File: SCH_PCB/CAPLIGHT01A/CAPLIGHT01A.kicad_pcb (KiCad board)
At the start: 2 copper layers, 76.2 x 20.3 mm, 25 parts, among them J1 JUMP_3X2, J10 JUMP_2x1, J11 JUMP_3X2, J5 CONN1_1, J6 CONN1_1, J9 JUMP_2x1, P1 USB_OTG, U1 LTC3625

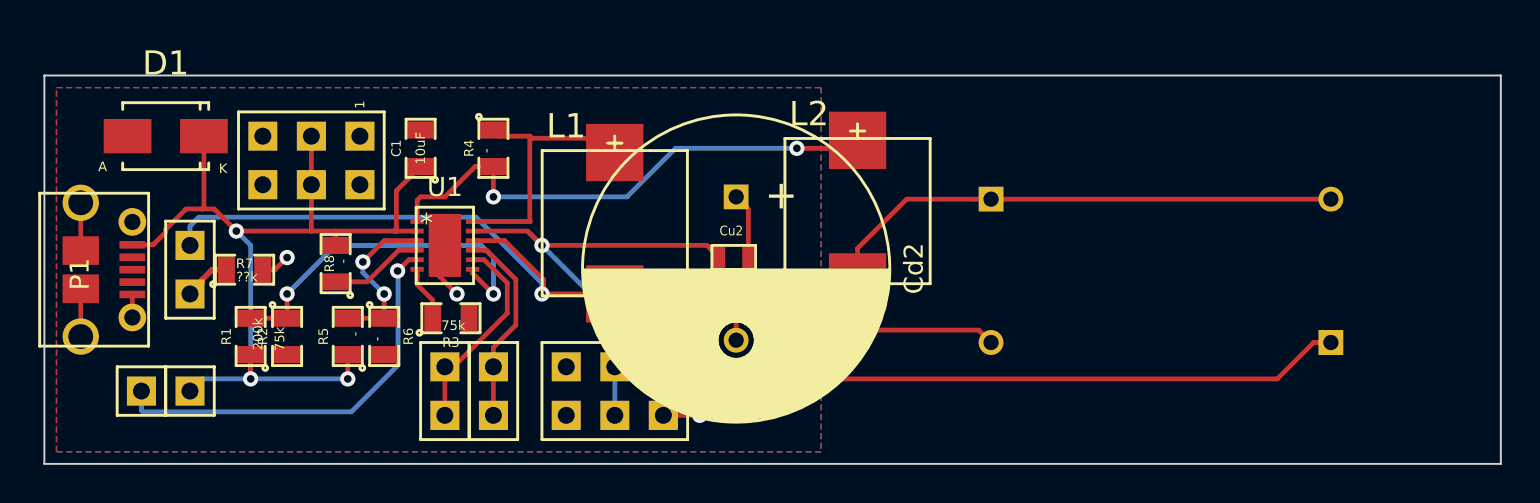
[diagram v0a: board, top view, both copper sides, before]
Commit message: only for ExpaLight
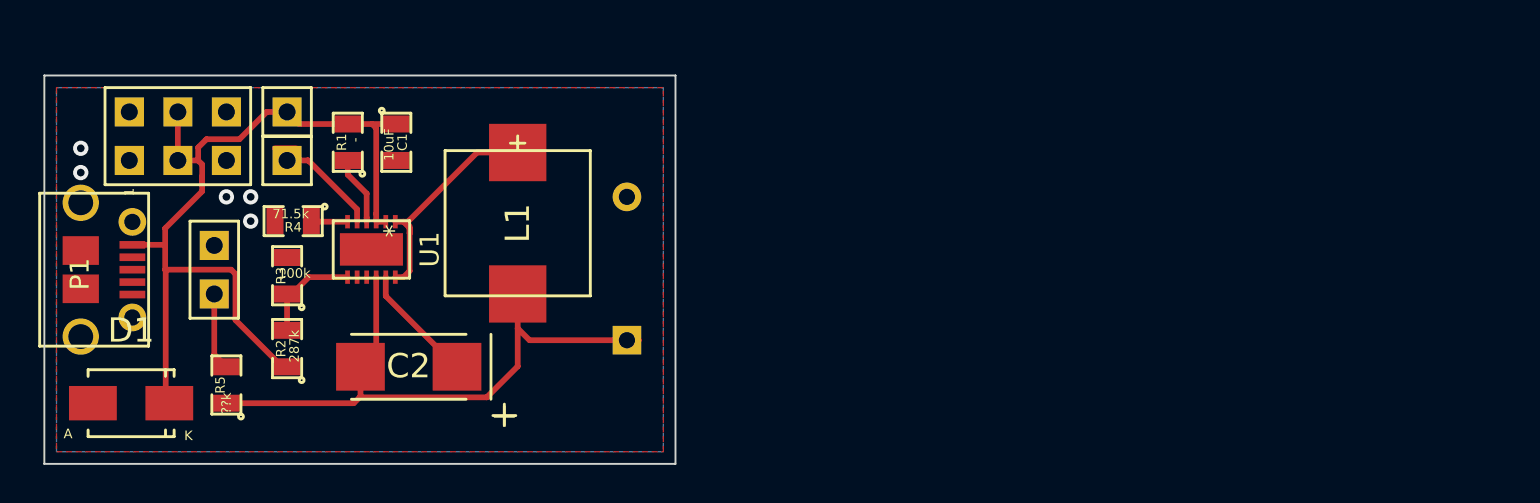
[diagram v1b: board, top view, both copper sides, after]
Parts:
- removed Cd1, Cd2, Cu1: 22F, Mlab_C:C_Radial_D16_L25_P7.5
- removed Cu2: 100uF, Mlab_C:SMD-0603
- removed J10, J9: JUMP_2x1, Mlab_Pin_Headers:Straight_2x01
- removed J11: JUMP_3X2, Mlab_Pin_Headers:Straight_2x03
- removed J5, J6: CONN1_1, Mlab_Pin_Headers:Straight_1x01
- removed L2: DER0705-3.3uH, Mlab_L:DER0705
- removed R6, R8: -, Mlab_R:SMD-0805
- removed R7: ??k, Mlab_R:SMD-0805
- added C2: 100uF, Mlab_C:TantalC_SizeC_Reflow, F.Cu at (156.9, 123.2)
- added C3: 22F, Mlab_C:C_Radial_D18_L25_P7.5, B.Cu at (168.3, 121.8)
- added J2: CONN1_1, Mlab_Pin_Headers:Straight_1x01, F.Cu at (150.5, 109.9)
- added J3: CONN1_1, Mlab_Pin_Headers:Straight_1x01, F.Cu at (150.5, 112.4)
- R1: value 200k -> -
- R2: value 75k -> 287k
- R3: value 75k -> 100k
- R4: value - -> 71.5k
- R5: value - -> ??k
- moved D1 14.1 mm to (142.3, 125.1)
- moved R1 11.4 mm to (153.7, 111.4)
- moved R4 11.1 mm to (150.8, 115.6), turned to 180 degrees
- moved R3 8.86 mm to (150.5, 118.4), turned to 90 degrees
- moved J1 7.10 mm to (144.8, 111.1), turned to 90 degrees
- moved R5 6.84 mm to (147.3, 124.1)
- moved L1 5.08 mm to (162.6, 115.7)
- moved U1 3.85 mm to (154.9, 117.0), turned to 270 degrees
- moved C1 1.31 mm to (156.2, 111.4), turned to 270 degrees
- moved D2 1.27 mm to (146.7, 118.1), turned to 0 degrees
- moved R2 0.63 mm to (150.5, 122.2), turned to 90 degrees
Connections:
- D2 pad 1: Net-(D2-Pad1) -> GND
- D2 pad 2: Net-(Cd1-Pad1) -> Net-(D2-Pad2)
- L1 pad 2: Net-(Cd1-Pad1) -> Net-(C2-Pad2)
- R1 pad 1: /VIN -> Net-(R1-Pad1)
- R1 pad 2: Net-(R1-Pad2) -> /VIN
- R2 pad 1: Net-(R1-Pad2) -> /VIN
- R2 pad 2: GND -> Net-(R2-Pad2)
- R3 pad 1: Net-(R3-Pad1) -> Net-(R2-Pad2)
- R4 pad 1: Net-(L1-Pad1) -> Net-(R4-Pad1)
- R4 pad 2: Net-(L2-Pad1) -> GND
- R5 pad 1: /VIN -> Net-(C2-Pad2)
- R5 pad 2: Net-(R5-Pad2) -> Net-(D2-Pad2)
- U1 pad 1: Net-(L2-Pad1) -> Net-(L1-Pad1)
- U1 pad 10: Net-(Cd1-Pad1) -> Net-(C2-Pad2)
- U1 pad 3: Net-(R5-Pad2) -> /VIN
- U1 pad 4: Net-(R8-Pad1) -> Net-(R1-Pad1)
- U1 pad 6: Net-(R3-Pad1) -> Net-(R4-Pad1)
- U1 pad 7: Net-(R1-Pad2) -> Net-(R2-Pad2)
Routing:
- net Net-(Cd1-Pad1): track 76.0 -> 0.00 mm, vias 1 -> 0
- net Net-(C2-Pad1): track 64.7 -> 6.25 mm, vias 2 -> 0
- net Net-(C2-Pad2): track 0.00 -> 33.0 mm
- net GND: track 29.8 -> 0.00 mm, vias 7 -> 5
- net Net-(L2-Pad1): track 27.7 -> 0.00 mm, vias 2 -> 0
- net Net-(R1-Pad2): track 18.9 -> 0.00 mm, vias 2 -> 0
- net /EN: track 21.7 -> 6.48 mm, vias 1 -> 0
- net /#PFO: track 10.9 -> 0.00 mm
- net /PG: track 10.5 -> 0.00 mm
- net Net-(R5-Pad2): track 8.82 -> 0.00 mm, vias 2 -> 0
- net Net-(R2-Pad2): track 0.00 -> 5.43 mm
- net Net-(R8-Pad1): track 4.95 -> 0.00 mm
- net Net-(D2-Pad2): track 0.00 -> 4.07 mm
- net Net-(R1-Pad1): track 0.00 -> 3.61 mm
- net Net-(R3-Pad1): track 2.90 -> 0.00 mm
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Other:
- board size 76.2 x 20.3 mm -> 33 x 20.3 mm
- board text removed: "#PFO"
- board text removed: "+"
- board text removed: "2016"
- board text removed: "CAPLIGHT01A"
- board text removed: "EN"
- board text removed: "LED"
- board text removed: "OUT"
- board text removed: "PG"
- board text removed: "Power IN"
